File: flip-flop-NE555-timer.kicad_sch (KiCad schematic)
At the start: 10 parts, among them J2 Conn_01x02_Pin, U1 NE555P

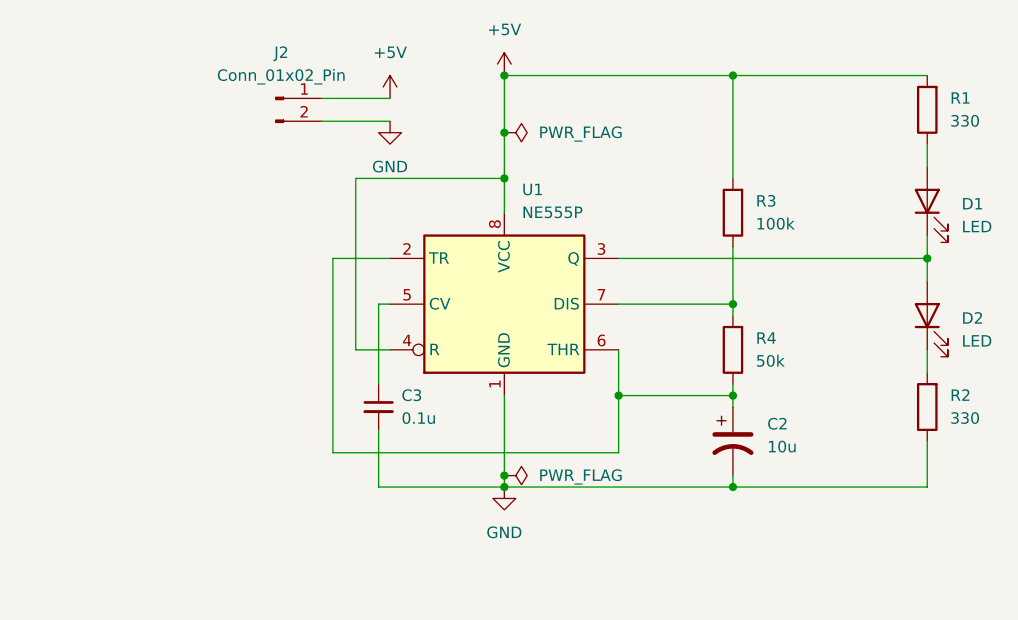
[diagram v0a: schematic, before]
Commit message: Add files via upload
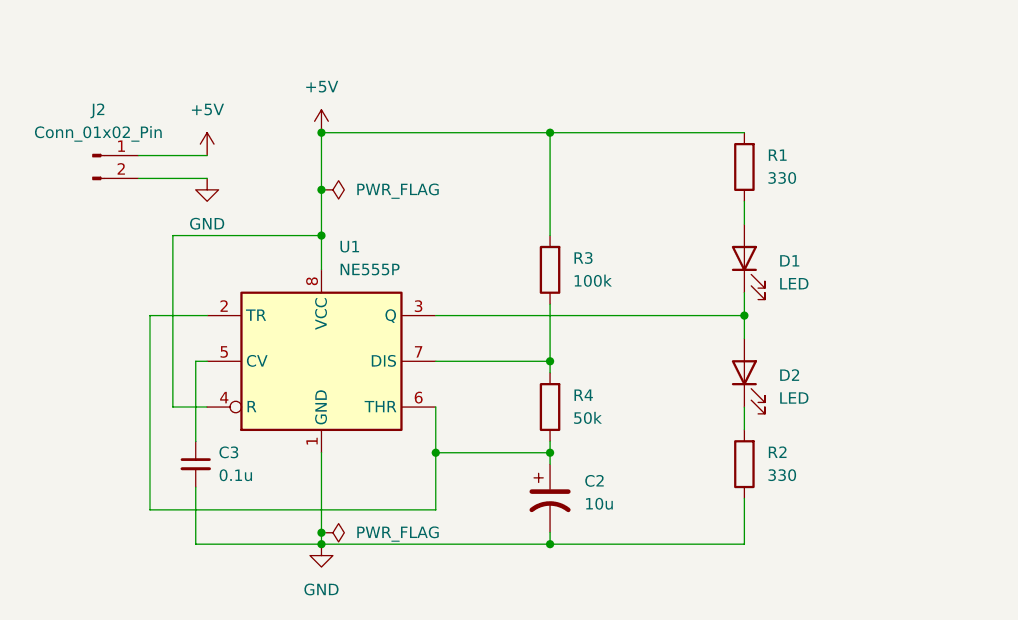
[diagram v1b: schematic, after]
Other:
- moved on the sheet: C2, C3, D1, D2, J2, R1, R2, R3, R4, U1
